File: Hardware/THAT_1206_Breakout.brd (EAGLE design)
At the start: 44.5 x 20.3 mm, 32 parts, among them IC1 THAT1206, J1 CHASSIS, J2 INPUT, J4 RN, J5 TN, J6 SN

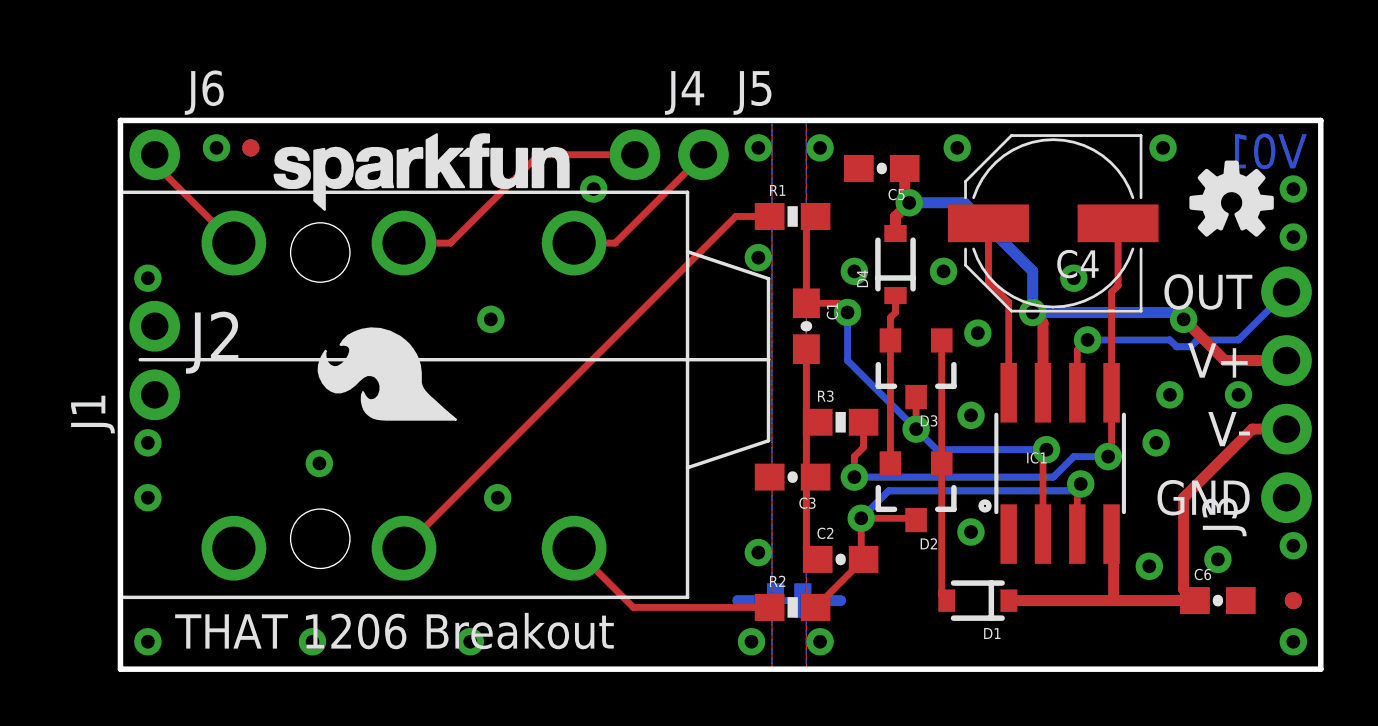
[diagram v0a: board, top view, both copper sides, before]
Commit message: Ran engineering checklist, a few small changes.
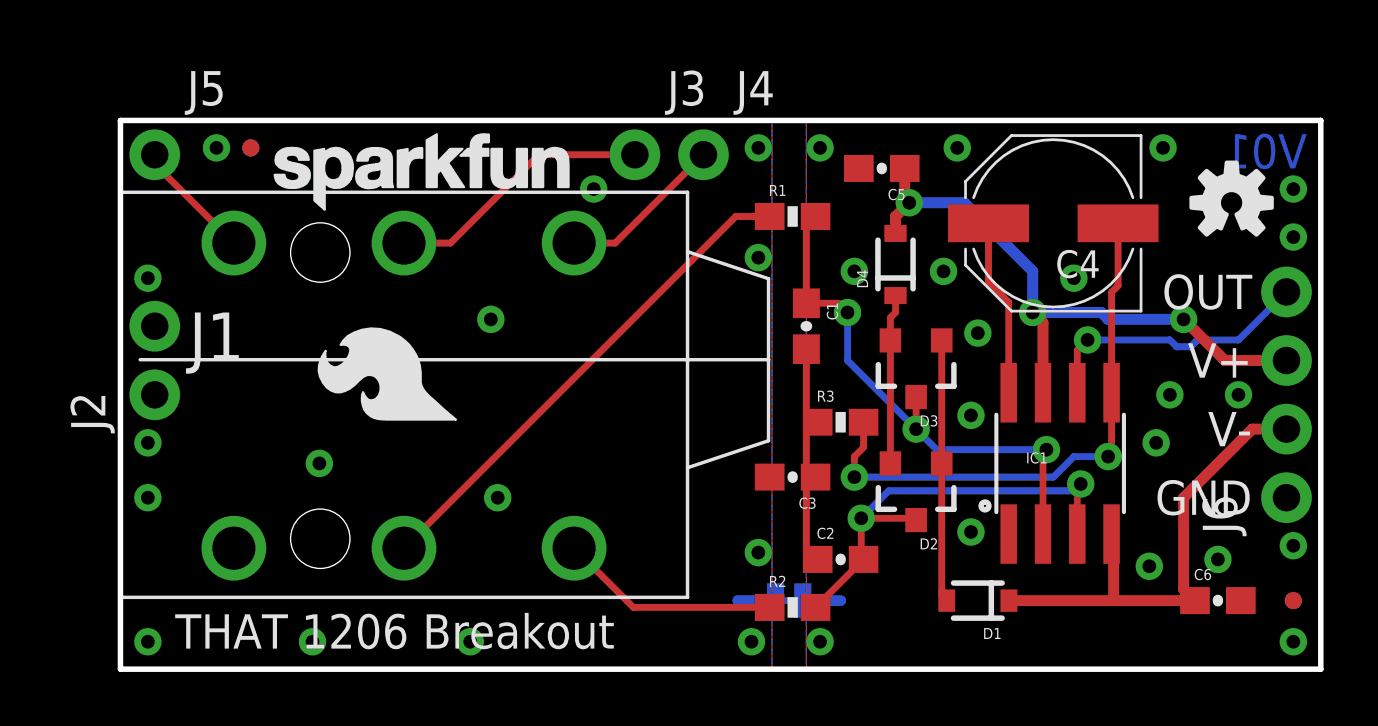
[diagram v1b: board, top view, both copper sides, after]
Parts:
- J1: value CHASSIS -> INPUT; device SparkFun-Connectors:1X02_NO_SILK -> SparkFun-Connectors:AUDIO-JACK-.25-INCH-HORIZ-PTH
- J2: value INPUT -> CHASSIS; device SparkFun-Connectors:AUDIO-JACK-.25-INCH-HORIZ-PTH -> SparkFun-Connectors:1X02_NO_SILK
- J3: value (none) -> RN; device SparkFun-Connectors:1X04_NO_SILK_ALL_ROUND -> SparkFun-Connectors:1X01_NO_SILK
- J4: value RN -> TN
- J5: value TN -> SN
- J6: value SN -> 1x4; device SparkFun-Connectors:1X01_NO_SILK -> SparkFun-Connectors:1X04_NO_SILK_ALL_ROUND
- LOGO2: value OSHW-LOGOS -> SFE_LOGO_FLAME.2_INCH; device SparkFun-Aesthetics:OSHW-LOGO-S -> SparkFun-Aesthetics:SFE_LOGO_FLAME_.2
- LOGO4: value SFE_LOGO_NAME.1_INCH -> OSHW-LOGOS; device SparkFun-Aesthetics:SFE_LOGO_NAME_.1 -> SparkFun-Aesthetics:OSHW-LOGO-S
- LOGO5: value SFE_LOGO_FLAME.2_INCH -> SFE_LOGO_NAME.1_INCH; device SparkFun-Aesthetics:SFE_LOGO_FLAME_.2 -> SparkFun-Aesthetics:SFE_LOGO_NAME_.1
- moved J6 43.8 mm to (43.2, 6.35), turned to 90 degrees
- moved FD1 42.1 mm to (43.4, 2.54), flipped to the bottom
- moved FD2 42.1 mm to (4.83, 19.3), flipped to the bottom, turned to 90 degrees
- moved FD3 42.1 mm to (4.83, 19.3), flipped to the top
- moved FD4 42.1 mm to (43.4, 2.54), flipped to the top, turned to 0 degrees
- moved LOGO4 35.9 mm to (41.1, 17.3)
- moved J3 27.3 mm to (19.1, 19.1), turned to 0 degrees
- moved LOGO2 24.6 mm to (12.7, 12.7), turned to 270 degrees
- moved J5 20.3 mm to (1.27, 19.1)
- moved LOGO5 8.41 mm to (5.21, 16.5), flipped to the top, turned to 0 degrees
- moved LOGO3 4.32 mm to (36.8, 17.3), flipped to the bottom
- moved J4 2.54 mm to (21.6, 19.1)
- moved J1 1.80 mm to (0.00, 11.4), turned to 0 degrees
- moved J2 1.80 mm to (1.27, 10.2), turned to 90 degrees
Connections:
- net GND: now also J6.1; no longer J3.1
- net GND-ISO: now also J1.SLEEVE, J2.1, J2.2; no longer J1.1, J1.2, J2.SLEEVE
- net N$1: now also J1.RING; no longer J2.RING
- net N$10: now also J1.RING-NORM, J3.1; no longer J2.RING-NORM, J4.1
- net N$3: now also J1.TIP; no longer J2.TIP
- net N$8: now also J1.SLEEVE-NORM, J5.1; no longer J2.SLEEVE-NORM, J6.1
- net N$9: now also J1.TIP-NORM, J4.1; no longer J2.TIP-NORM, J5.1
- net RCV: now also J6.4; no longer J3.4
- net VCC: now also J6.3; no longer J3.3
- net VNEG: now also J6.2; no longer J3.2
